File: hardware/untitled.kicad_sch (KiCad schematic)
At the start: 2 parts

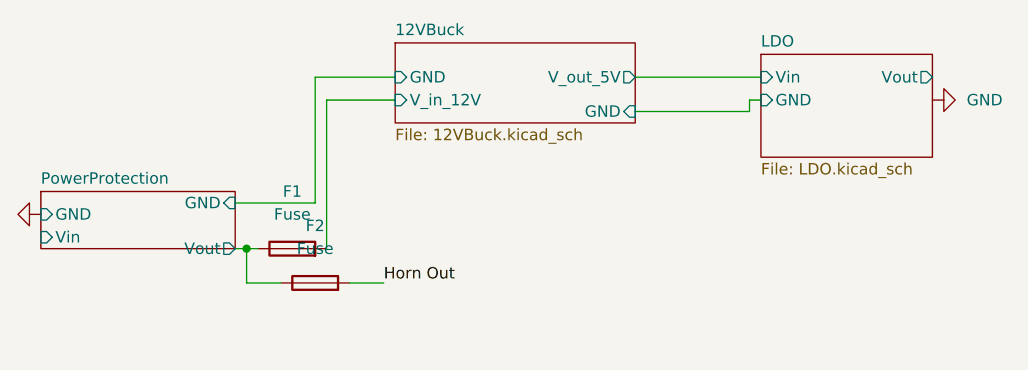
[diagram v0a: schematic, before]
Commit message: mcu and power
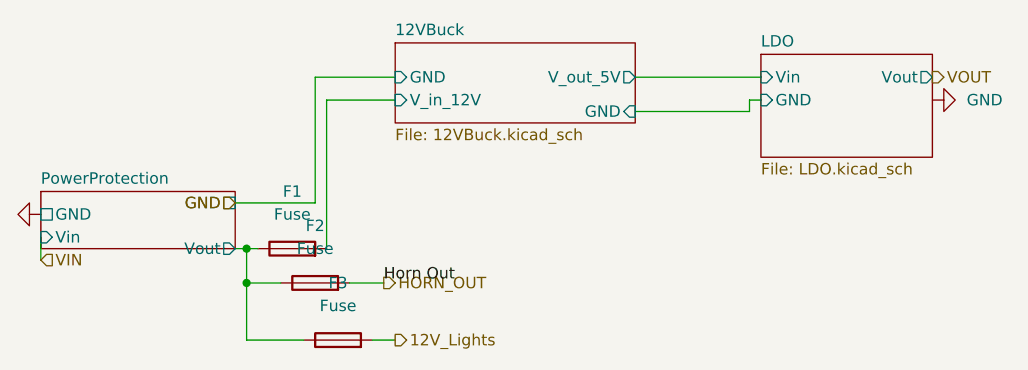
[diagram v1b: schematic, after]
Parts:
- added F3: Fuse, symbol Device:Fuse
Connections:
- net PowerProtection/Vout: now also F3.1
- net Horn Out renamed HORN_OUT
- new net 12V_Lights: F3.2
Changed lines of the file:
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@@
 		(color 0 0 0 0)
 	)
+	(junction
+		(at 100.33 52.07)
+		(diameter 0)
+		(color 0 0 0 0)
+	)
 	(wire
 		(pts
@@
 	(wire
 		(pts
+			(xy 77.47 46.99) (xy 77.47 49.53)
+		)
+		(stroke
+			(width 0)
+			(type default)
+		)
+	)
+	(wire
+		(pts
 			(xy 107.95 29.21) (xy 116.84 29.21)
 		)
@@
 	(wire
 		(pts
+			(xy 100.33 52.07) (xy 100.33 58.42)
+		)
+		(stroke
+			(width 0)
+			(type default)
+		)
+	)
+	(wire
+		(pts
 			(xy 100.33 48.26) (xy 101.6 48.26)
+		)
+		(stroke
+			(width 0)
+			(type default)
+		)
+	)
+	(wire
+		(pts
+			(xy 114.3 58.42) (xy 116.84 58.42)
+		)
+		(stroke
+			(width 0)
+			(type default)
+		)
+	)
+	(wire
+		(pts
+			(xy 100.33 58.42) (xy 106.68 58.42)
 		)
 		(stroke
@@
 			)
 			(justify left bottom)
+		)
+	)
+	(hierarchical_label "GND"
+		(shape input)
+		(at 99.06 43.18 180)
+		(effects
+			(font
+				(size 1.27 1.27)
+			)
+			(justify right)
+		)
+	)
+	(hierarchical_label "12V_Lights"
+		(shape output)
+		(at 116.84 58.42 0)
+		(effects
+			(font
+				(size 1.27 1.27)
+			)
+			(justify left)
+		)
+	)
+	(hierarchical_label "VIN"
+		(shape input)
+		(at 77.47 49.53 0)
+		(effects
+			(font
+				(size 1.27 1.27)
+			)
+			(justify left)
+		)
+	)
+	(hierarchical_label "VOUT"
+		(shape output)
+		(at 176.53 29.21 0)
+		(effects
+			(font
+				(size 1.27 1.27)
+			)
+			(justify left)
+		)
+	)
+	(hierarchical_label "HORN_OUT"
+		(shape output)
+		(at 115.57 52.07 0)
+		(effects
+			(font
+				(size 1.27 1.27)
+			)
+			(justify left)
 		)
 	)
@@
 	(symbol
 		(lib_id "Device:Fuse")
+		(at 110.49 58.42 90)
+		(unit 1)
+		(body_style 1)
+		(exclude_from_sim no)
+		(in_bom yes)
+		(on_board yes)
+		(in_pos_files yes)
+		(dnp no)
+		(fields_autoplaced yes)
+		(property "Reference" "F3"
+			(at 110.49 52.07 90)
+			(show_name no)
+			(do_not_autoplace no)
+			(effects
+				(font
+					(size 1.27 1.27)
+				)
+			)
+		)
+		(property "Value" "Fuse"
+			(at 110.49 54.61 90)
+			(show_name no)
+			(do_not_autoplace no)
+			(effects
+				(font
+					(size 1.27 1.27)
+				)
+			)
+		)
+		(property "Footprint" ""
+			(at 110.49 60.198 90)
+			(hide yes)
+			(show_name no)
+			(do_not_autoplace no)
+			(effects
+				(font
+					(size 1.27 1.27)
+				)
+			)
+		)
+		(property "Datasheet" ""
+			(at 110.49 58.42 0)
+			(hide yes)
+			(show_name no)
+			(do_not_autoplace no)
+			(effects
+				(font
+					(size 1.27 1.27)
+				)
+			)
+		)
+		(property "Description" "Fuse"
+			(at 110.49 58.42 0)
+			(hide yes)
+			(show_name no)
+			(do_not_autoplace no)
+			(effects
+				(font
+					(size 1.27 1.27)
+				)
+			)
+		)
+		(pin "2"
+		)
+		(pin "1"
+		)
+		(instances
+			(project "DEI"
+				(path "/1469f349-54e5-4a37-953e-ac48c70e29b2/d41a835d-0002-40e6-b2c5-562251bf7d32"
+					(reference "F3")
+					(unit 1)
+				)
+			)
+		)
+	)
+	(symbol
+		(lib_id "Device:Fuse")
 		(at 105.41 48.26 90)
 		(unit 1)
@@
 			)
 		)
-		(pin "GND" input
+		(pin "GND" passive
 			(at 77.47 44.45 180)
 			(effects
@@
 			)
 		)
-		(pin "GND" input
+		(pin "GND" passive
 			(at 99.06 43.18 0)
 			(effects
